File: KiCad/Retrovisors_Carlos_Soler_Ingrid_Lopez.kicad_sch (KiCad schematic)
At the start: 1 part, among them U1 LM74700

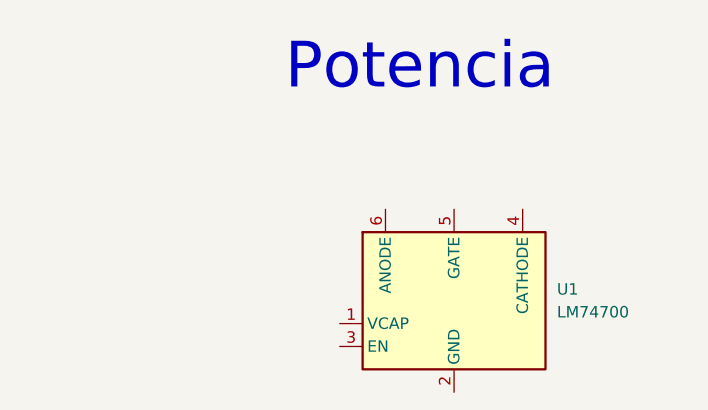
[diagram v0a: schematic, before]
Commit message: Etapa de alimentació 1
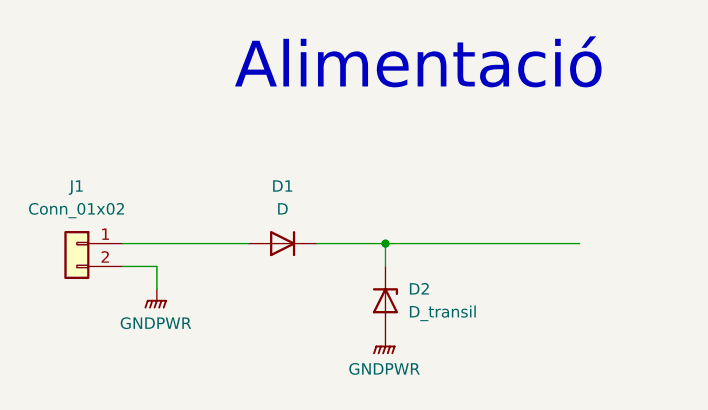
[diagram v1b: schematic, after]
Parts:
- removed U1: LM74700, Package_TO_SOT_SMD:SOT-23-6, symbol Power_Management:LM74700
- added D1: D, symbol Device:D
- added D2: D_transil, symbol Device:D_Zener
- added J1: Conn_01x02, symbol Connector_Generic:Conn_01x02
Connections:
- new net: D1.2 (A), J1.1 (Pin_1)
- new net: D1.1 (K), D2.1 (K)
- new net GNDPWR: D2.2 (A), J1.2 (Pin_2)
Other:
- note added: "Alimentació"
- note removed: "Potencia"
